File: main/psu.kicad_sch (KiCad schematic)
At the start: 34 parts, among them U201 TSV911xxLx, U202 LMR51430, U203 LDK130M33R, U204 LM317_SOT-223

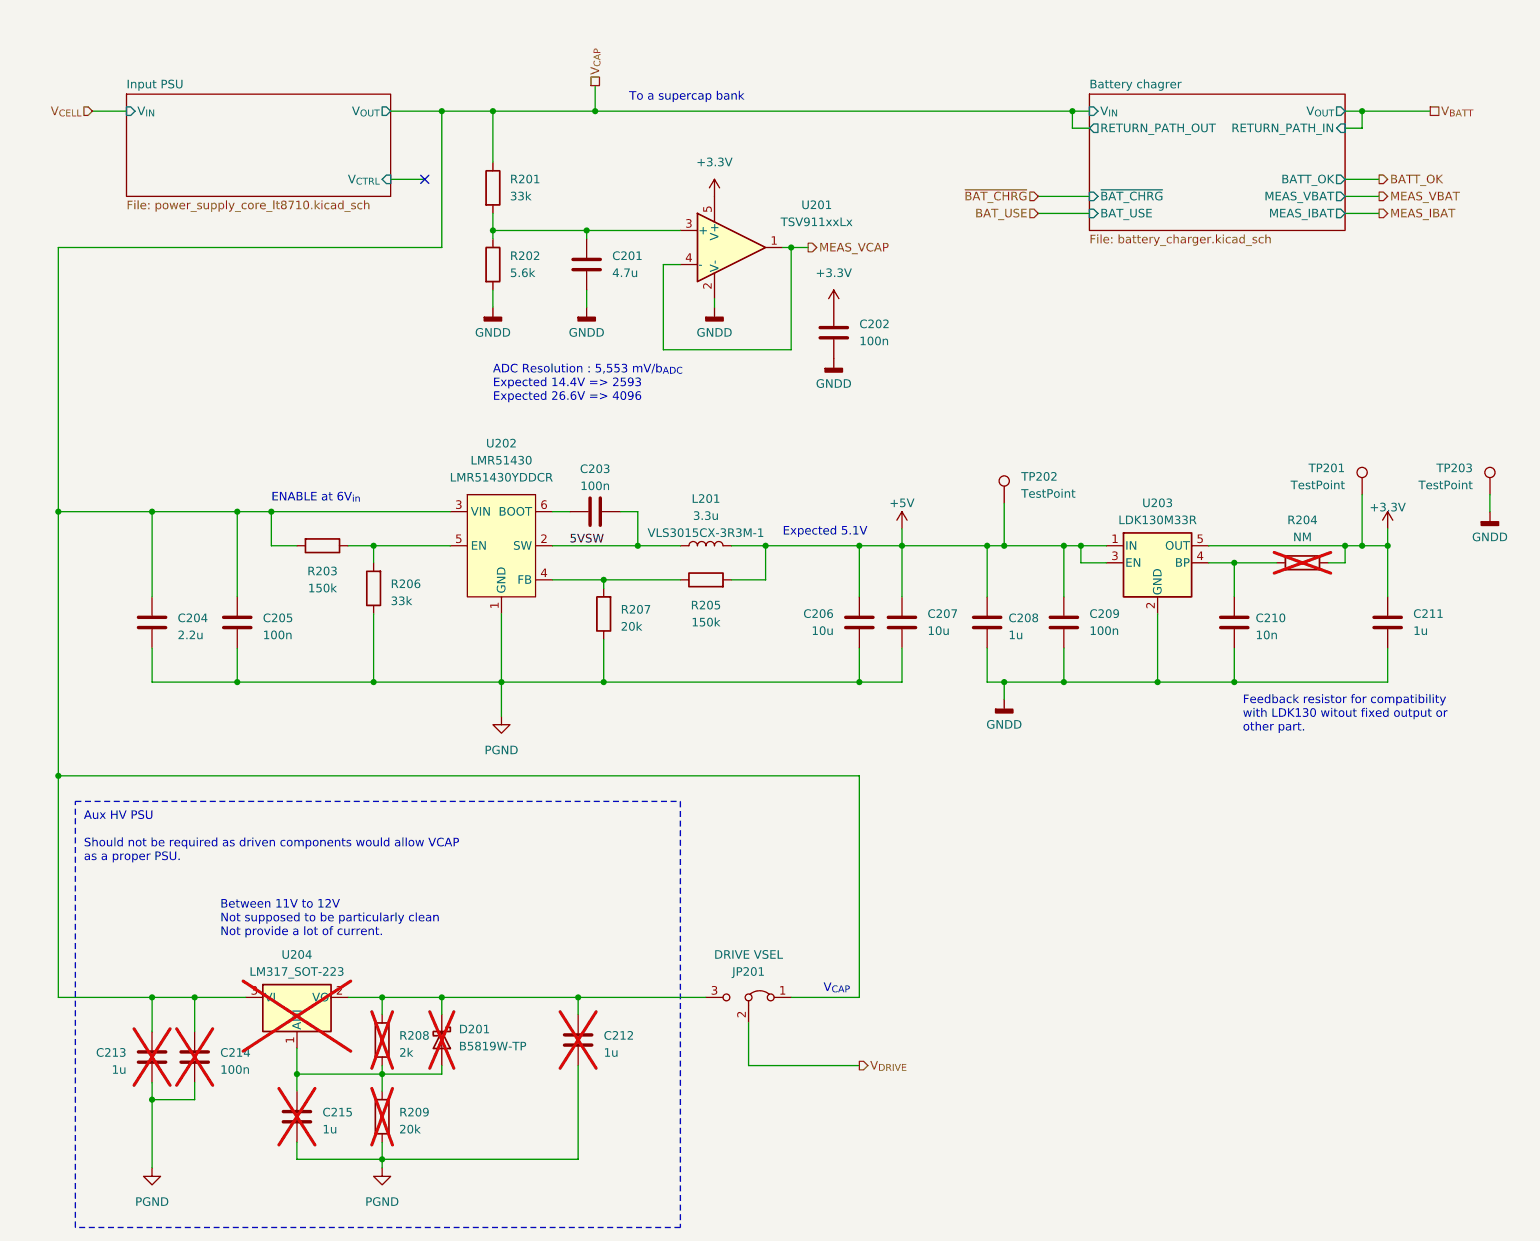
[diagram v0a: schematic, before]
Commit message: Sent to fab
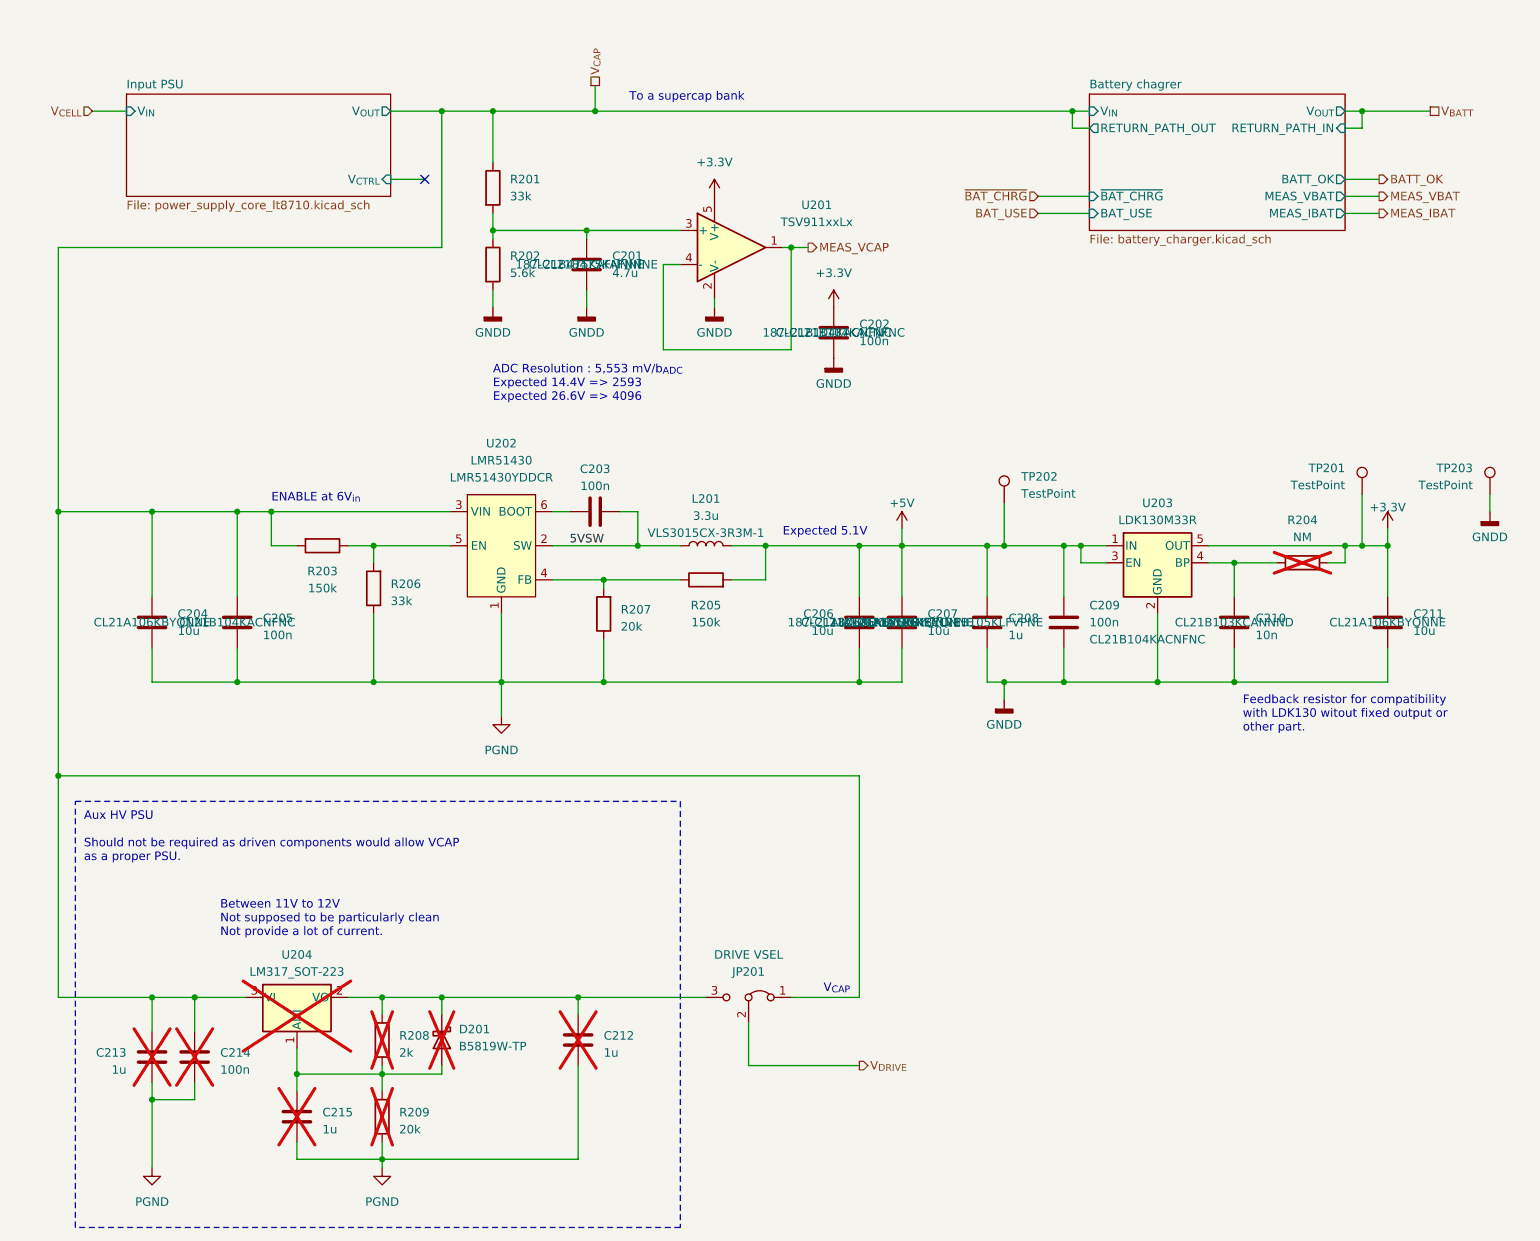
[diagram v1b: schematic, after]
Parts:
- C201: MPN (none) -> CL21B475KAFNNNE; Mouser SKU (none) -> 187-CL21B475KAFNNNE
- C202, C205, C209: MPN (none) -> CL21B104KACNFNC; Mouser SKU (none) -> 187-CL21B104KACNFNC
- C203: MPN 0805YC104M4T2A -> CL21B104KACNFNC; Mouser SKU 581-0805YC104M4T2A -> 187-CL21B104KACNFNC
- C204: value 2.2u -> 10u; MPN (none) -> CL21A106KBYQNNE; Mouser SKU (none) -> 187-CL21A106KBYQNNE
- C206, C207: MPN (none) -> CL21A106KBYQNNE; Mouser SKU (none) -> 187-CL21A106KBYQNNE
- C208: MPN (none) -> CL21B105KLFVPNE; Mouser SKU (none) -> 187-CL21B105KLFVPNE
- C210: MPN (none) -> CL21B103KCANNND; Mouser SKU (none) -> 187-CL21B103KCANNND
- C211: value 1u -> 10u; MPN (none) -> CL21A106KBYQNNE; Mouser SKU (none) -> 187-CL21A106KBYQNNE
